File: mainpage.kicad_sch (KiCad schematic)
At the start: 0 parts

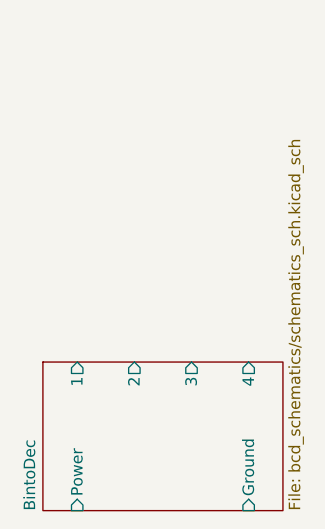
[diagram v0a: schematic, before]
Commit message: 9th Button Schematics
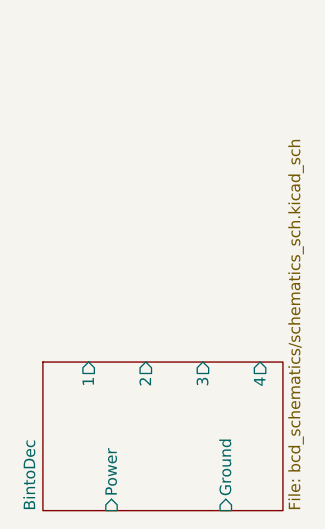
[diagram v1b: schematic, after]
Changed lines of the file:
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@@
-			)
-		)
-		(pin "Power" input
-			(at 130.81 143.51 270)
-			(effects
-				(font
-					(size 1.27 1.27)
-				)
-				(justify left)
 			)
 		)
 		(pin "1" output
-			(at 130.81 127 90)
+			(at 132.08 127 90)
 			(effects
 				(font
@@
 		)
 		(pin "2" output
-			(at 137.16 127 90)
+			(at 138.43 127 90)
 			(effects
 				(font
@@
 		)
 		(pin "3" output
-			(at 143.51 127 90)
+			(at 144.78 127 90)
 			(effects
 				(font
@@
 		)
 		(pin "4" output
-			(at 149.86 127 90)
+			(at 151.13 127 90)
 			(effects
 				(font
@@
 		)
 		(pin "Ground" input
-			(at 149.86 143.51 270)
+			(at 147.32 143.51 270)
 			(effects
 				(font
+					(size 1.27 1.27)
+				)
+				(justify left)
+			)
+		)
+		(pin "Power" input
+			(at 134.62 143.51 270)
+			(effects
+				(font
